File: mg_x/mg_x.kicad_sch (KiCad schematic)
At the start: 15 parts, among them IC1 TC118S, J1 Conn_01x02, J2 Conn_01x03, J3 Conn_01x03, U1 ATtiny88-A, U2 AMS1117-3.3, U3 MCP4561-502E_MS, U4 ACS712xLCTR-05B, U5 MPU-6050

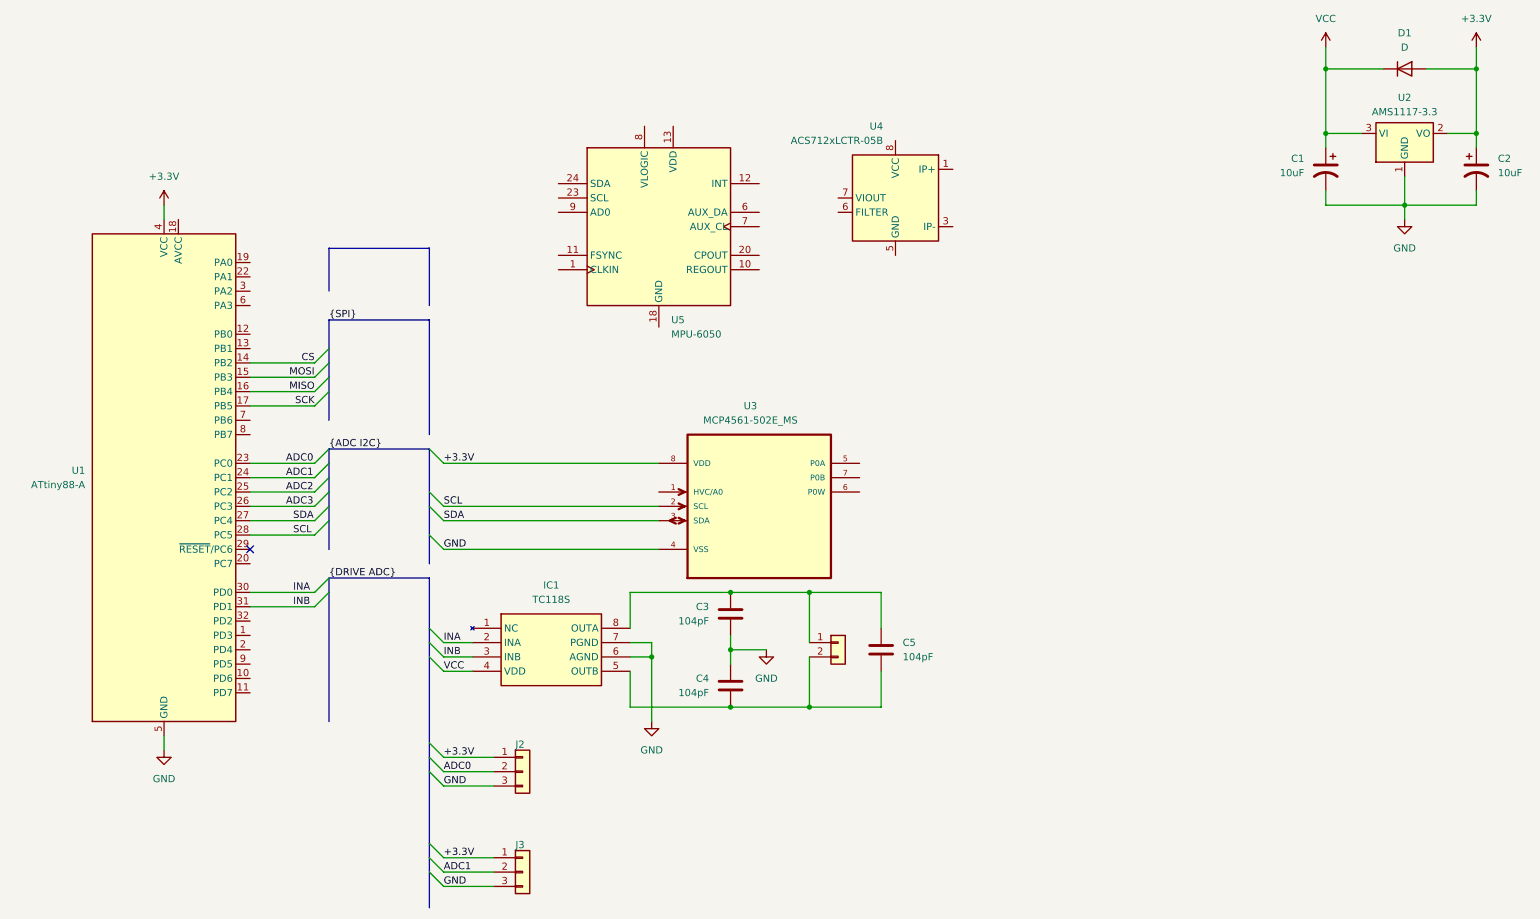
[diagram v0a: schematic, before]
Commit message: Improved MG-X
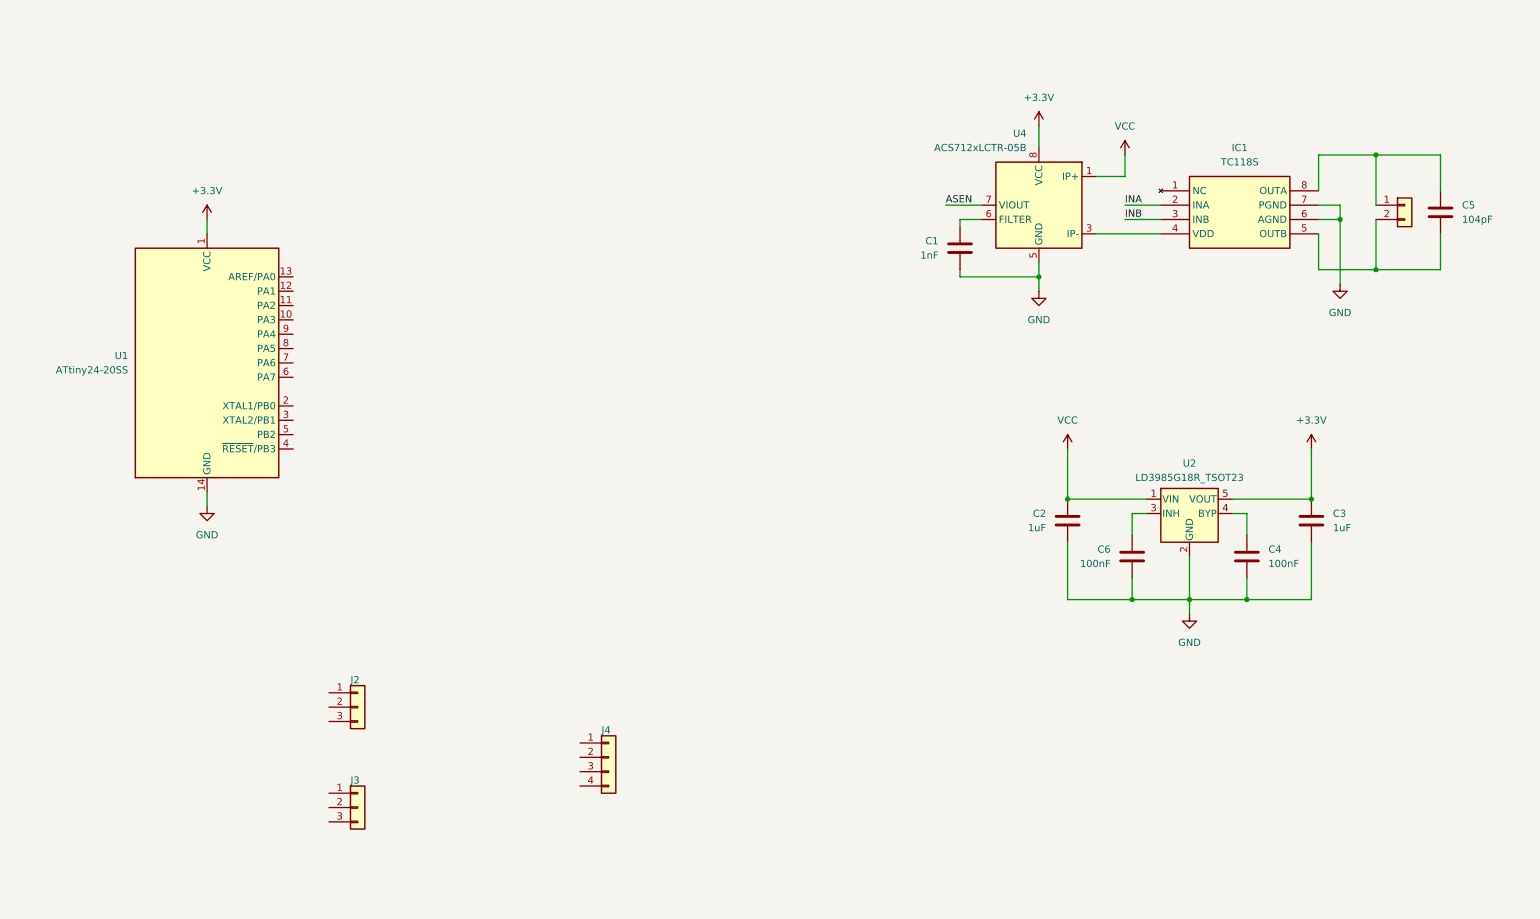
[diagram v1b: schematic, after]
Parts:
- removed C1, C2: 10uF, symbol Device:C_Polarized_US
- removed D1: D, symbol Device:D
- removed U1: ATtiny88-A, Package_QFP:TQFP-32_7x7mm_P0.8mm, symbol MCU_Microchip_ATtiny:ATtiny88-A
- removed U2: AMS1117-3.3, Package_TO_SOT_SMD:SOT-223-3_TabPin2, symbol Regulator_Linear:AMS1117-3.3
- removed U3: MCP4561-502E_MS, MCP4561-502E_MS:SOP65P490X110-8N, symbol MCP4561-502E_MS:MCP4561-502E_MS
- removed U5: MPU-6050, Sensor_Motion:InvenSense_QFN-24_4x4mm_P0.5mm, symbol Sensor_Motion:MPU-6050
- added C1: 1nF, Capacitor_SMD:C_1206_3216Metric, symbol Device:C
- added C2: 1uF, Capacitor_SMD:C_1206_3216Metric, symbol Device:C
- added C6: 100nF, Capacitor_SMD:C_0402_1005Metric, symbol Device:C
- added J4: Conn_01x04, symbol Connector_Generic:Conn_01x04
- added U1: ATtiny24-20SS, Package_SO:SOIC-14_3.9x8.7mm_P1.27mm, symbol MCU_Microchip_ATtiny:ATtiny24-20SS
- added U2: LD3985G18R_TSOT23, Package_TO_SOT_SMD:TSOT-23-5, symbol Regulator_Linear:LD3985G18R_TSOT23
- C3: value 104pF -> 1uF; footprint (none) -> Capacitor_SMD:C_1206_3216Metric
- C4: value 104pF -> 100nF; footprint (none) -> Capacitor_SMD:C_0402_1005Metric
- C5: footprint (none) -> Capacitor_SMD:C_1206_3216Metric
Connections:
- net +3.3V: now also C3.1, U4.8 (VCC), U1.1 (VCC), U2.5 (VOUT); no longer J2.1 (Pin_1), J3.1 (Pin_1)
- net GND: now also C4.2, U4.5 (GND), C1.2, C2.2, C6.2, U1.14 (GND), U2.2 (GND); no longer C4.1, J2.3 (Pin_3), J3.3 (Pin_3)
- net VCC: now also U4.1 (IP+), U4.2 (IP+), C2.1, U2.1 (VIN); no longer IC1.4 (VDD)
- net at U4.3 (IP-), U4.4 (IP-): now also IC1.4 (VDD)
- net at U4.6 (FILTER): now also C1.1
- net ASEN: now reaches U4.7 (VIOUT)
- net at C5.1, IC1.8 (OUTA), J1.1 (Pin_1): no longer C3.1
- net at C5.2, IC1.5 (OUTB), J1.2 (Pin_2): no longer C4.2
- net ADC0: no longer names the net of J2.2 (Pin_2)
- net ADC1: no longer names the net of J3.2 (Pin_2)
- new net: C4.1, U2.4 (BYP)
- new net: C6.1, U2.3 (INH)
- no-connect marks 1 -> 0
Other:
- moved on the sheet: C5, IC1, J2, J3, U4
